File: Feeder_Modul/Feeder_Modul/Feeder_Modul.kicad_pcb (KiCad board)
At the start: 2 copper layers, 156.6 x 125.2 mm, 89 parts, among them J1 Conn_02x01, J101 Conn_02x01, J102 Conn_01x06_Male, J103 Conn_02x01, J104 Conn_02x01, J105 Conn_02x01, J106 USB_A, J107 Conn_02x07_Odd_Even, J108 Conn_02x01, Q101 BC847, SW101 SW_Push, SW102 SW_Push, SW103 SW_Push, SW104 SW_Push, SW105 SW_Push, U1 TPS560430, U101 TPS560430, U102 STM32F105R8Tx, U103 M24C01-WMN, U104 EE-SX1350_PCB, U105 DRV8835, U107 SN65HVD230, Y101 48MHz

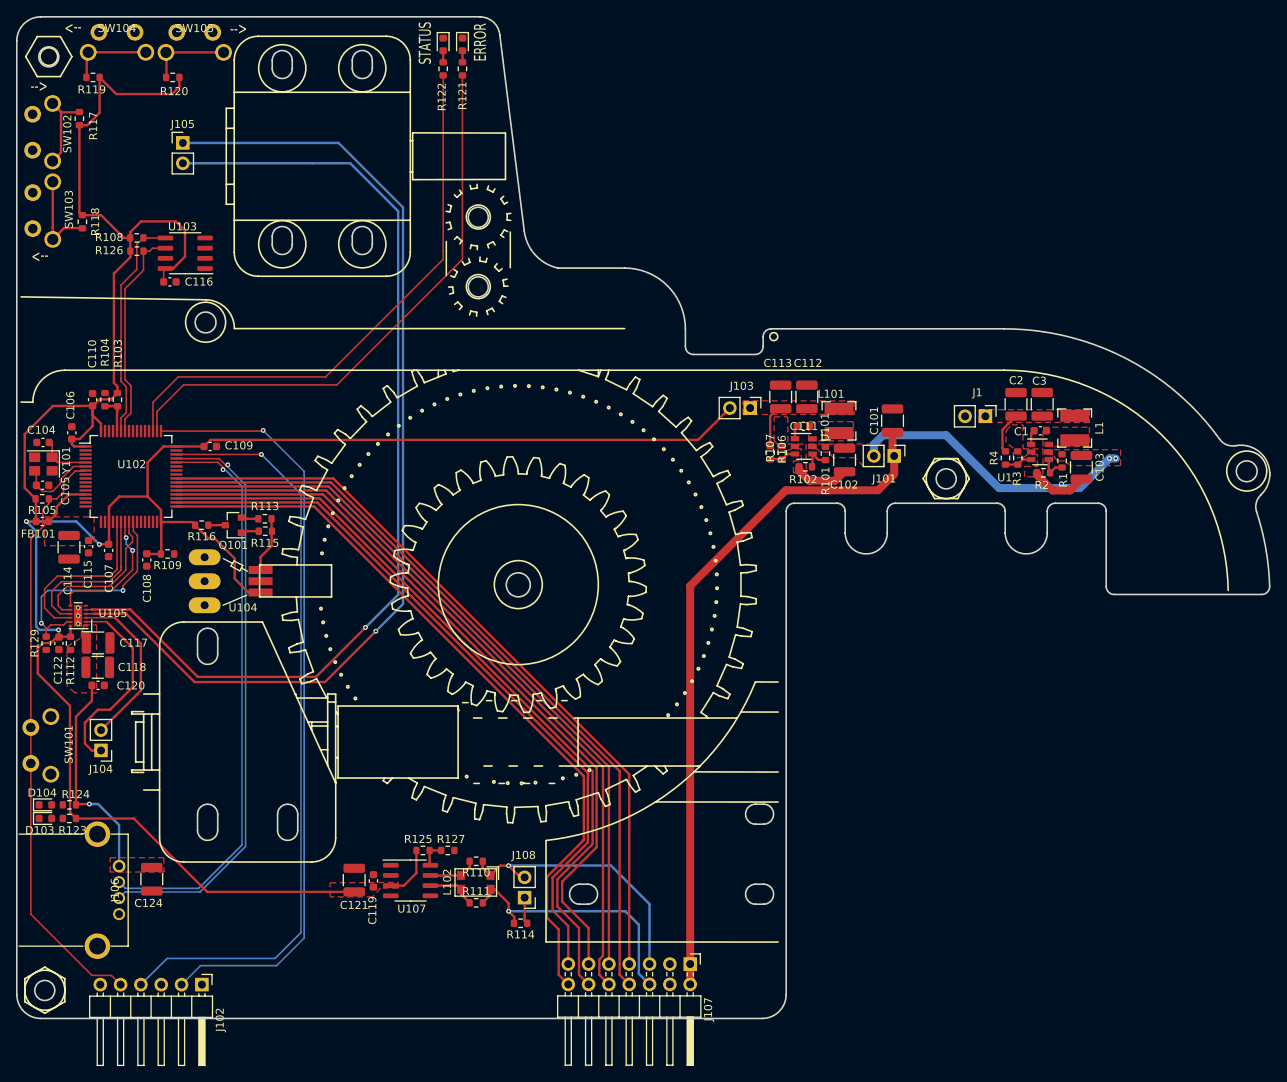
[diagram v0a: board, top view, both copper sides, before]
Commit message: Feeder fertig
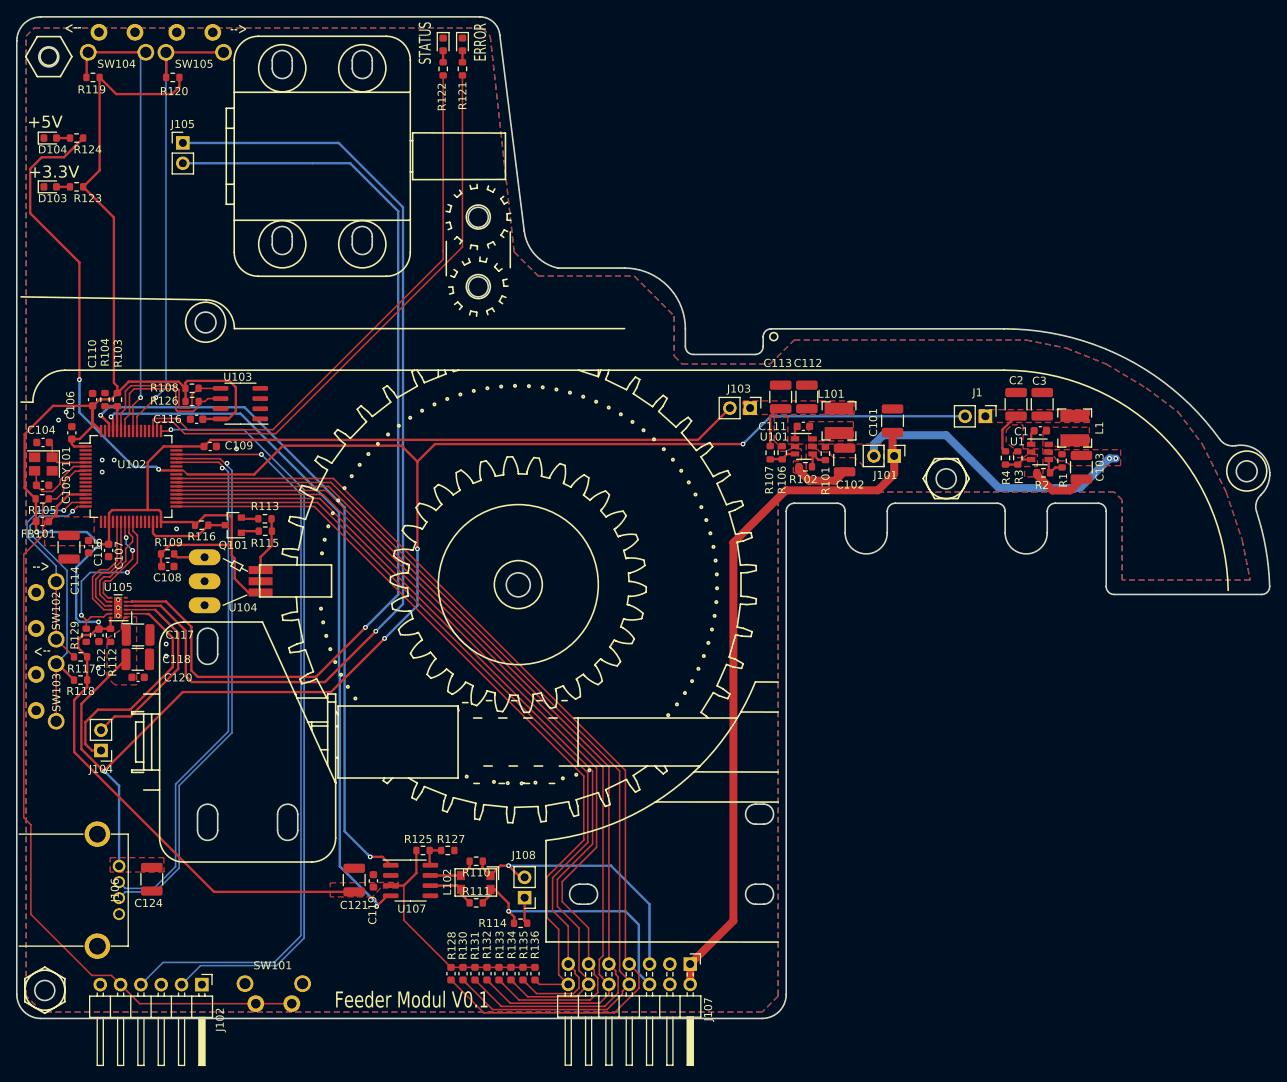
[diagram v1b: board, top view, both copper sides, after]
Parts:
- added R128: 88K7, Resistor_SMD:R_0603_1608Metric, F.Cu at (118.1, 155.2)
- added R130: 88K7, Resistor_SMD:R_0603_1608Metric, F.Cu at (119.6, 155.2)
- added R131: 88K7, Resistor_SMD:R_0603_1608Metric, F.Cu at (121.1, 155.2)
- added R132: 88K7, Resistor_SMD:R_0603_1608Metric, F.Cu at (122.6, 155.2)
- added R133: 88K7, Resistor_SMD:R_0603_1608Metric, F.Cu at (124.1, 155.2)
- added R134: 88K7, Resistor_SMD:R_0603_1608Metric, F.Cu at (125.6, 155.2)
- added R135: 88K7, Resistor_SMD:R_0603_1608Metric, F.Cu at (127.1, 155.2)
- added R136: 88K7, Resistor_SMD:R_0603_1608Metric, F.Cu at (128.6, 155.2)
- R112: value 0R -> DNP
- moved R124 83.4 mm to (71.3, 50.8)
- moved D104 83.4 mm to (68.0, 50.8)
- moved R123 79.0 mm to (71.3, 56.9)
- moved D103 79.0 mm to (68.0, 56.9)
- moved R117 67.3 mm to (71.8, 115.6), turned to 0 degrees
- moved SW103 60.2 mm to (66.2, 120.0)
- moved SW102 59.8 mm to (66.2, 109.8)
- moved R118 57.3 mm to (71.8, 118.5), turned to 0 degrees
- moved SW101 44.3 mm to (96.0, 158.9), turned to 0 degrees
- moved R126 20.0 mm to (85.7, 83.7)
- moved R108 20.0 mm to (85.7, 82.0)
- moved U103 20.0 mm to (91.8, 84.0)
- moved C116 17.5 mm to (86.3, 85.9), turned to 180 degrees
- moved C117 5.10 mm to (79.0, 112.9)
- moved C118 5.10 mm to (78.9, 115.9)
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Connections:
- J102 pad 6: Net-(J102-Pad6) -> (no net)
- U102 pad 10: Net-(U102-Pad10) -> (no net)
- U102 pad 11: Net-(U102-Pad11) -> (no net)
- U102 pad 14: Net-(U102-Pad14) -> (no net)
- U102 pad 15: Net-(U102-Pad15) -> /BTN_TBACK
- U102 pad 16: Net-(U102-Pad16) -> /BTN_TFOR
- U102 pad 17: Net-(U102-Pad17) -> (no net)
- U102 pad 2: Net-(U102-Pad2) -> (no net)
- U102 pad 20: Net-(U102-Pad20) -> (no net)
- U102 pad 26: Net-(U102-Pad26) -> (no net)
- U102 pad 27: Net-(U102-Pad27) -> (no net)
- U102 pad 28: Net-(U102-Pad28) -> (no net)
- U102 pad 29: Net-(U102-Pad29) -> (no net)
- U102 pad 3: Net-(U102-Pad3) -> (no net)
- U102 pad 30: Net-(U102-Pad30) -> /ENC_OUT
- U102 pad 4: Net-(U102-Pad4) -> (no net)
- U102 pad 41: /PA8 -> (no net)
- U102 pad 43: /PA10 -> (no net)
- U102 pad 52: Net-(U102-Pad52) -> (no net)
- U102 pad 53: Net-(U102-Pad53) -> (no net)
- U102 pad 54: Net-(U102-Pad54) -> (no net)
- U102 pad 55: Net-(U102-Pad55) -> /BTN_SFOR
- U102 pad 56: Net-(U102-Pad56) -> /BTN_SBACK
- U102 pad 57: Net-(U102-Pad57) -> (no net)
- U102 pad 8: Net-(U102-Pad8) -> (no net)
- U102 pad 9: Net-(U102-Pad9) -> (no net)
- U104 pad 2: Net-(U104-Pad2) -> (no net)
- U104 pad 5: Net-(U104-Pad5) -> (no net)
- U107 pad 5: Net-(U107-Pad5) -> (no net)
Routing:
- net +5V: track 27.4 -> 255.9 mm, vias 1 -> 6
- net /CAN1_RX: track 0.00 -> 89.2 mm, vias 0 -> 2
- net /CAN1_TX: track 0.00 -> 86.5 mm, vias 0 -> 2
- net /BTN_SFOR: track 10.4 -> 59.2 mm, vias 0 -> 1
- net /BTN_SBACK: track 10.4 -> 58.4 mm, vias 0 -> 1
- net /ADDR0: track 95.6 -> 125.6 mm
- net +3V3: track 334.0 -> 361.6 mm
- net /BTN_TFOR: track 11.5 -> 38.2 mm, vias 0 -> 1
- net /ADDR2: track 93.2 -> 117.3 mm
- net /ADDR1: track 97.5 -> 121.3 mm
- net /NRST: track 74.5 -> 97.6 mm
- net /ADDR3: track 95.5 -> 113.6 mm
- net /ADDR4: track 94.3 -> 112.1 mm
- net /BTN_TBACK: track 11.9 -> 27.6 mm, vias 0 -> 1
- net /ADDR6: track 91.9 -> 103.5 mm
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- added copper zone on B.Cu, net GND
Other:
- board text added: "+3.3V"
- board text added: "+5V"
- board text added: "Feeder Modul V0.1"
